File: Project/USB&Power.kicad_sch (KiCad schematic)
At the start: 12 parts, among them J1 JST SH, J2 Pico EZmate, J2 USB_C sink board 1.3mm, U58 PRTR5V0U2X

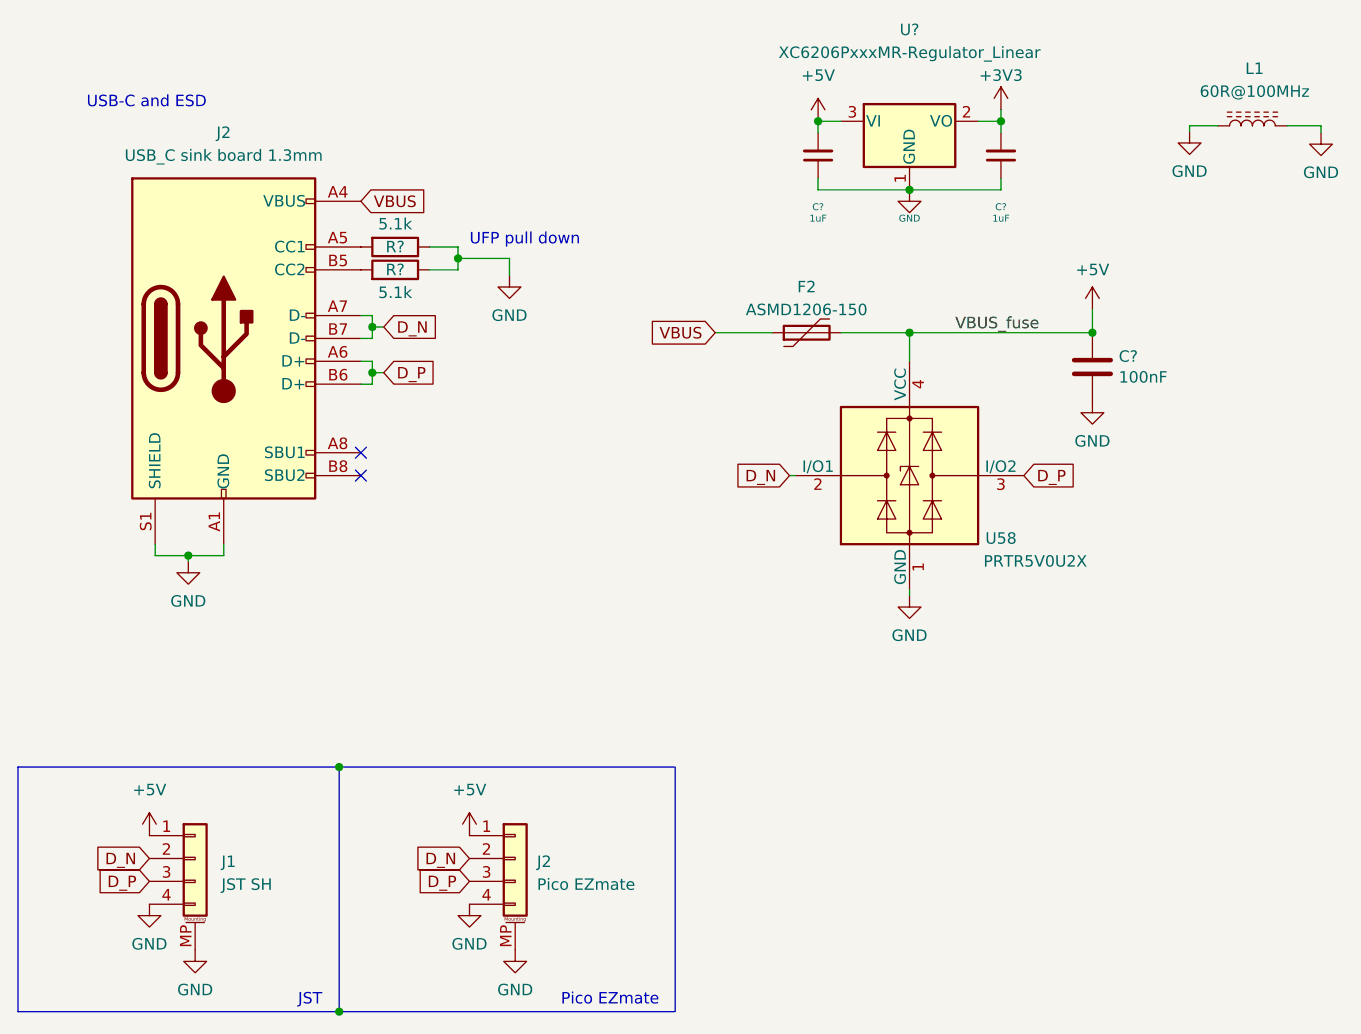
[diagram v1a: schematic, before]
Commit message: pin revision
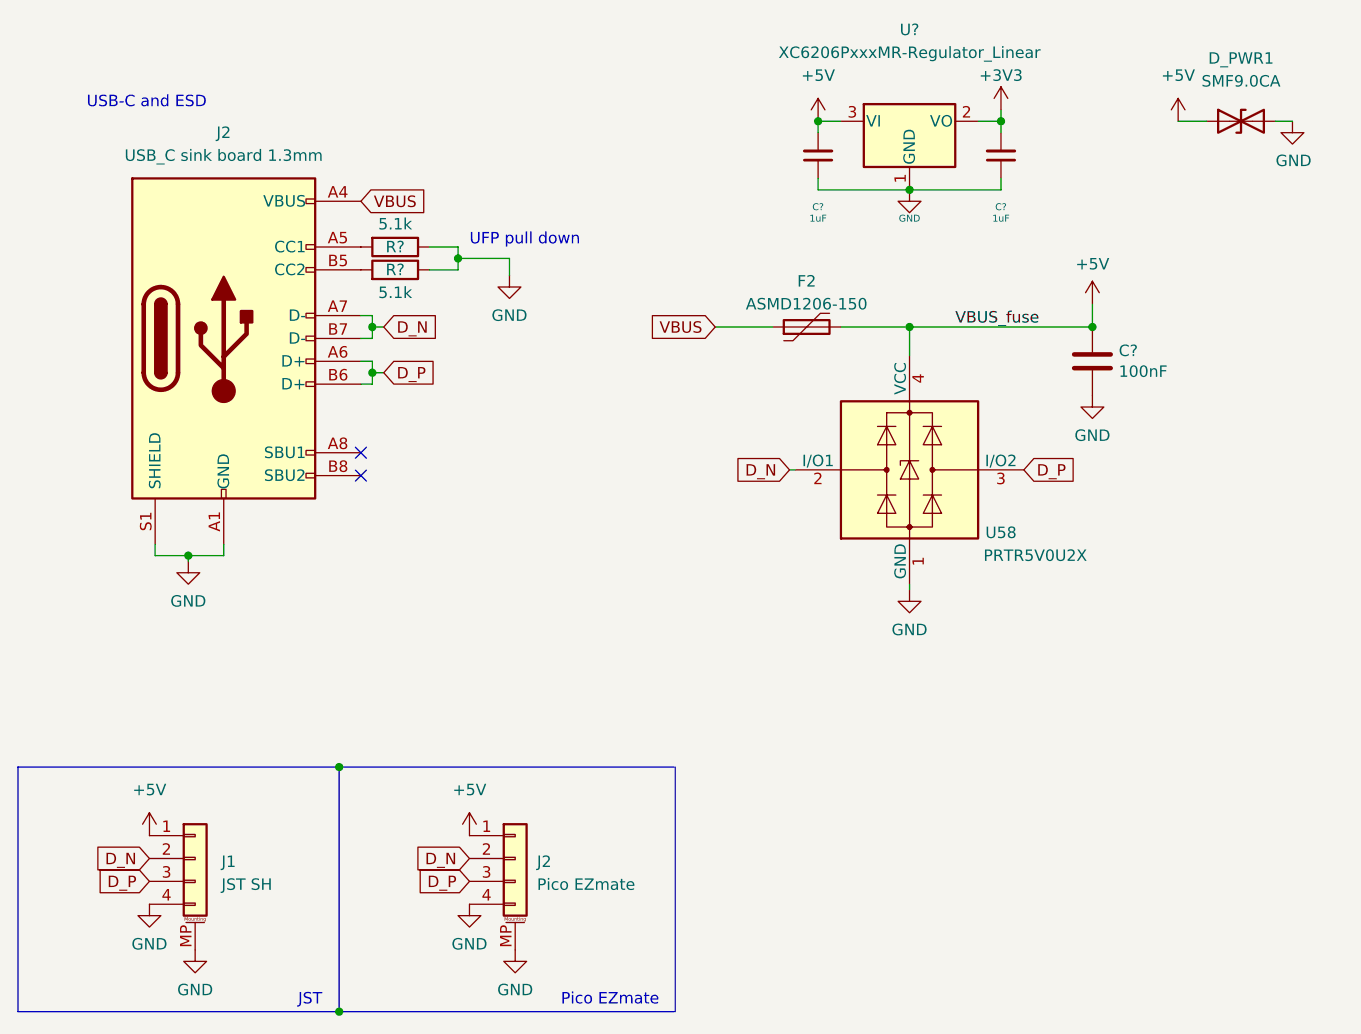
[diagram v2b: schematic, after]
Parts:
- removed L1: 60R@100MHz, Inductor_SMD:L_1206_3216Metric, symbol Unified-Daughterboard-rescue:L_Core_Ferrite-Device
- added D_PWR1: SMF9.0CA, Diode_SMD:D_SOD-123, symbol Device:D_TVS
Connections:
- net +5V: now also D_PWR1.1 (A1)
- net GND: now also D_PWR1.2 (A2)
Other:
- moved on the sheet: C?, F2, U58
